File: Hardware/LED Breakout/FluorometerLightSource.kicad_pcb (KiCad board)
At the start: 2 copper layers, 50.8 x 50.8 mm, 14 parts, among them Q1 BSS214NW, Q2 BSS214NW, Q3 BSS214NW, Q4 BSS214NW

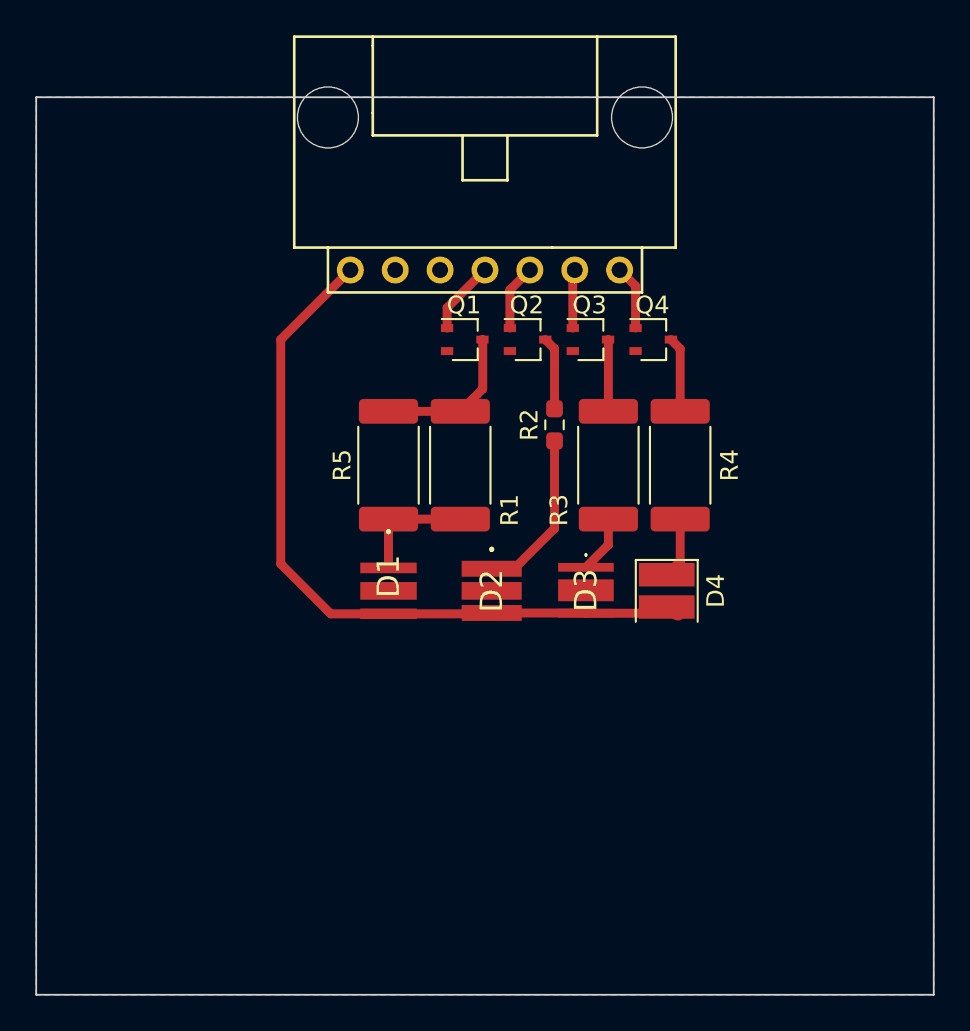
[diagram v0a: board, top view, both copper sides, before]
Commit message: Breakout Boards
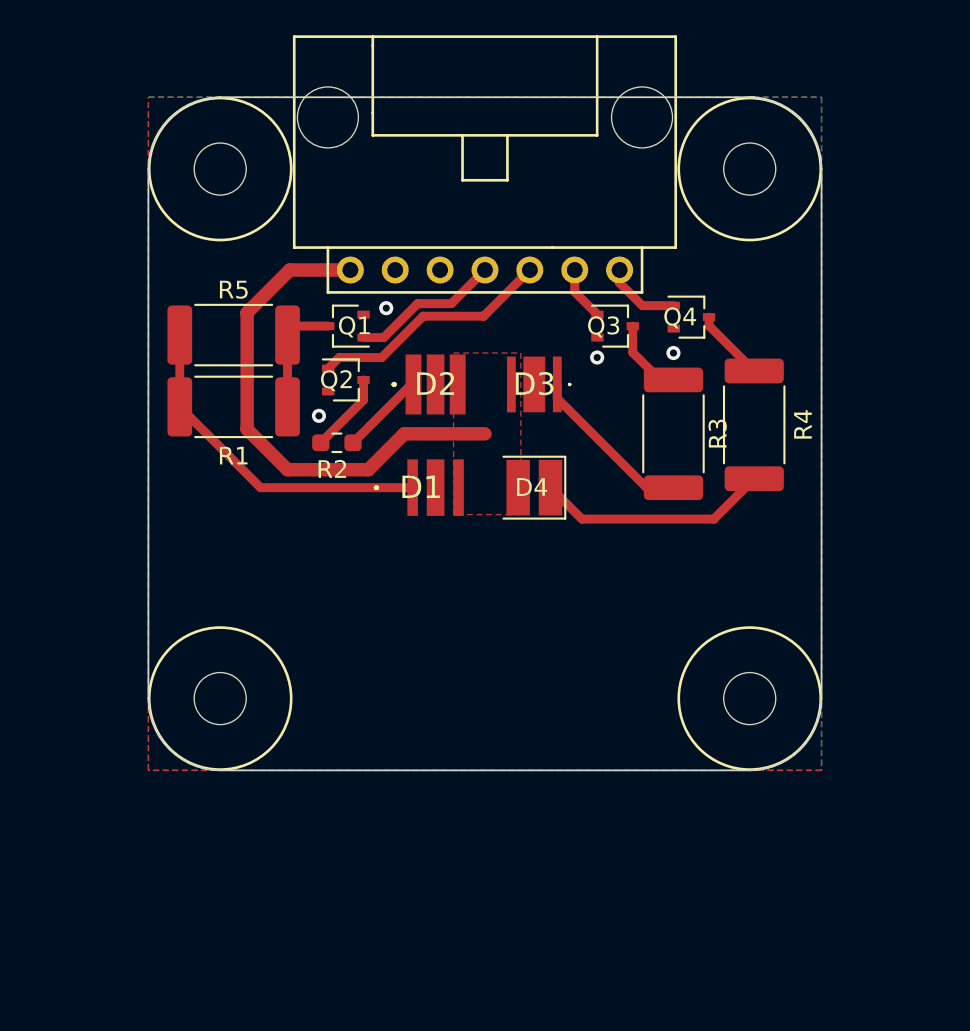
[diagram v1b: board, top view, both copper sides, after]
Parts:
- added V1: Via, MRDT_Drill_Holes:4_40_Hole, F.Cu at (109.5, 74.9)
- added V2: Via, MRDT_Drill_Holes:4_40_Hole, F.Cu at (109.5, 104.9)
- added V3: Via, MRDT_Drill_Holes:4_40_Hole, F.Cu at (79.5, 74.9)
- added V4: Via, MRDT_Drill_Holes:4_40_Hole, F.Cu at (79.5, 104.9)
- moved D3 13.3 mm to (96.2, 87.1), turned to 180 degrees
- moved R1 13.2 mm to (80.3, 88.4), turned to 0 degrees
- moved R2 12.4 mm to (86.1, 90.4), turned to 180 degrees
- moved D2 12.1 mm to (91.7, 87.1), turned to 0 degrees
- moved R5 11.4 mm to (80.3, 84.3), turned to 0 degrees
- moved Q2 10.5 mm to (86.6, 86.9)
- moved D4 9.50 mm to (97.3, 93.0), turned to 180 degrees
- moved Q1 6.77 mm to (86.6, 83.8), turned to 180 degrees
- moved D1 6.42 mm to (91.7, 93.0), turned to 0 degrees
- moved R4 4.77 mm to (109.7, 89.4)
- moved R3 4.09 mm to (105.2, 89.9)
- moved Q4 2.50 mm to (106.2, 83.3)
- moved Q3 1.59 mm to (101.9, 83.8)
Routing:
- net +12V: track 42.2 -> 28.7 mm
- net Net-(D1-Pad1): track 6.83 -> 19.1 mm
- net Net-(Conn1-Pad5): track 3.75 -> 13.7 mm
- net Net-(D4-Pad1): track 3.46 -> 13.2 mm
- net Net-(D3-Pad1): track 3.25 -> 9.46 mm
- net Net-(D2-Pad1): track 9.45 -> 4.79 mm
- net Net-(Conn1-Pad4): track 4.17 -> 8.46 mm
- net Net-(Q1-Pad3): track 8.66 -> 6.57 mm
- net Net-(Conn1-Pad7): track 3.66 -> 4.33 mm
- net GND: vias 0 -> 4
- added copper zone on F.Cu, net +12V
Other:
- board size 50.8 x 50.8 mm -> 38.1 x 38.1 mm
